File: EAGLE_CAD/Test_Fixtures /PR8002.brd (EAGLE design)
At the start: 118.5 x 99.3 mm, 59 parts, among them J1 M3_SCREW_POST

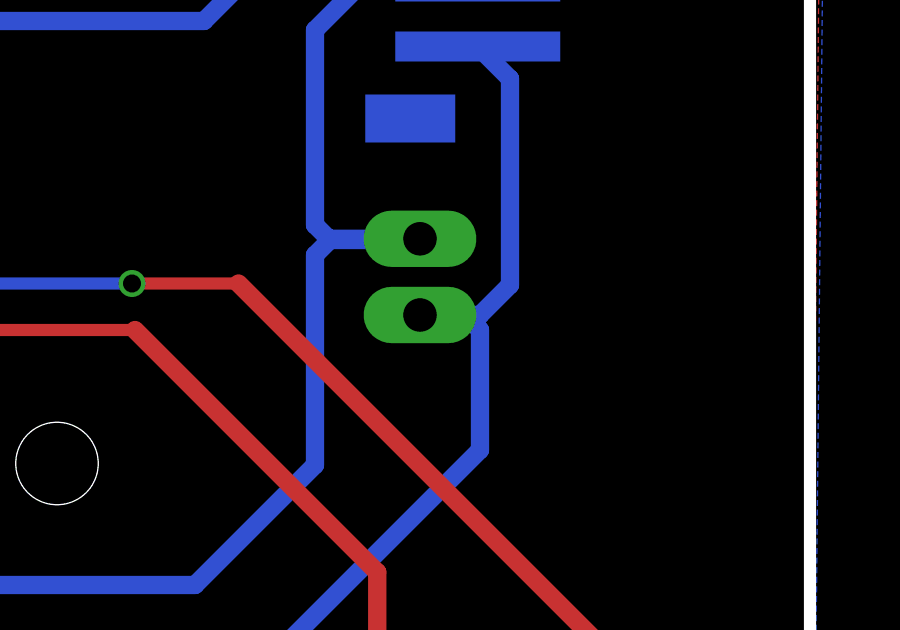
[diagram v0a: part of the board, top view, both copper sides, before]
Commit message: Updates to PR8002
Updates to PR8002
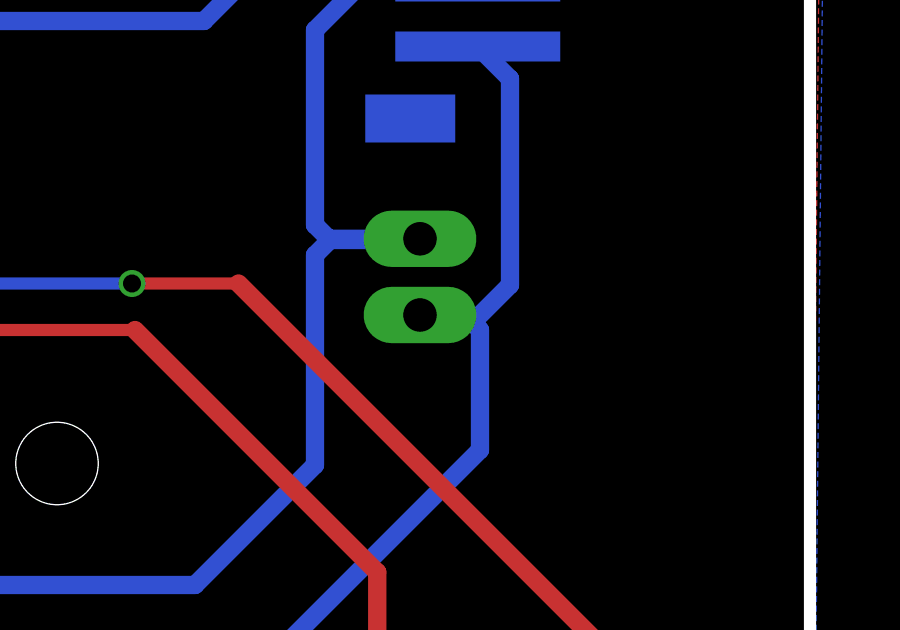
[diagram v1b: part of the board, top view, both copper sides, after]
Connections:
- net SPK_OUT-: no longer JP2.1
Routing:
- net SPK_OUT-: track 79.8 -> 76.3 mm
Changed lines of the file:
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@@
 <wire x1="100.3" y1="18.8" x2="108" y2="26.5" width="0.6096" layer="16"/>
 <wire x1="108" y1="39.875" x2="107.925" y2="39.95" width="0.6096" layer="16"/>
-<contactref element="JP2" pad="1"/>
 <wire x1="108" y1="26.5" x2="108" y2="30.5" width="0.6096" layer="16"/>
 <wire x1="108" y1="30.5" x2="107.5" y2="31" width="0.6096" layer="16"/>
-<wire x1="107.5" y1="31" x2="106" y2="31" width="0.6096" layer="16"/>
-<wire x1="106" y1="31" x2="108" y2="31" width="0.6096" layer="16"/>
 <wire x1="108" y1="31" x2="109" y2="32" width="0.6096" layer="16"/>
 <wire x1="109" y1="32" x2="109" y2="38.875" width="0.6096" layer="16"/>
 <wire x1="109" y1="38.875" x2="107.925" y2="39.95" width="0.6096" layer="16"/>
+<wire x1="108" y1="30.5" x2="108" y2="31" width="0" layer="19" extent="16-16"/>
 </signal>
 <signal name="MISO">
